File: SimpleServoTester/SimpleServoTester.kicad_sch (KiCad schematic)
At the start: 41 parts, among them J2 Servo, J2 USBASP, J3 OLED, Q1 IRLZ44N, SW1 POWER, SW2 RotaryEncoder_Switch, U1 ATmega328-A, U2 LM7805_TO220, U3 INA219AxD, U4 AMS1117-3.3, Y2 16MHz

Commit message: update
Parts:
- removed C10: 100n/50V, Capacitor_SMD:C_0603_1608Metric, symbol Device:C_Small
- removed RV1: 10k, Footprint:PTV09A-4225F-B502, symbol Device:R_Potentiometer
- added C7, C8: 100n/50V, Capacitor_SMD:C_0603_1608Metric, symbol Device:C_Small
- added R10, R8: 100R, Resistor_SMD:R_0603_1608Metric, symbol Device:R_Small
- H1, H2, H3, H4: footprint MountingHole:MountingHole_3.2mm_M3_Pad_Via -> MountingHole:MountingHole_3.2mm_M3
- SW2: footprint (none) -> Rotary_Encoder:RotaryEncoder_Alps_EC11E-Switch_Vertical_H20mm
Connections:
- net GND: now also SW2.C, C7.1, C8.2
- net at SW2.A: now also R8.2
- net at SW2.B: now also R10.2
- net INT_PIN_2: now reaches U1.1 (PD3)
- net INT_PIN_2: now also C7.2, R8.1
- net DI: now reaches U1.2 (PD4)
- net DI: now also C8.1, R10.1
- no-connect marks 14 -> 12
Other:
- note removed: "POTENTIOMETER"
- moved on the sheet: C15, R9, SW2

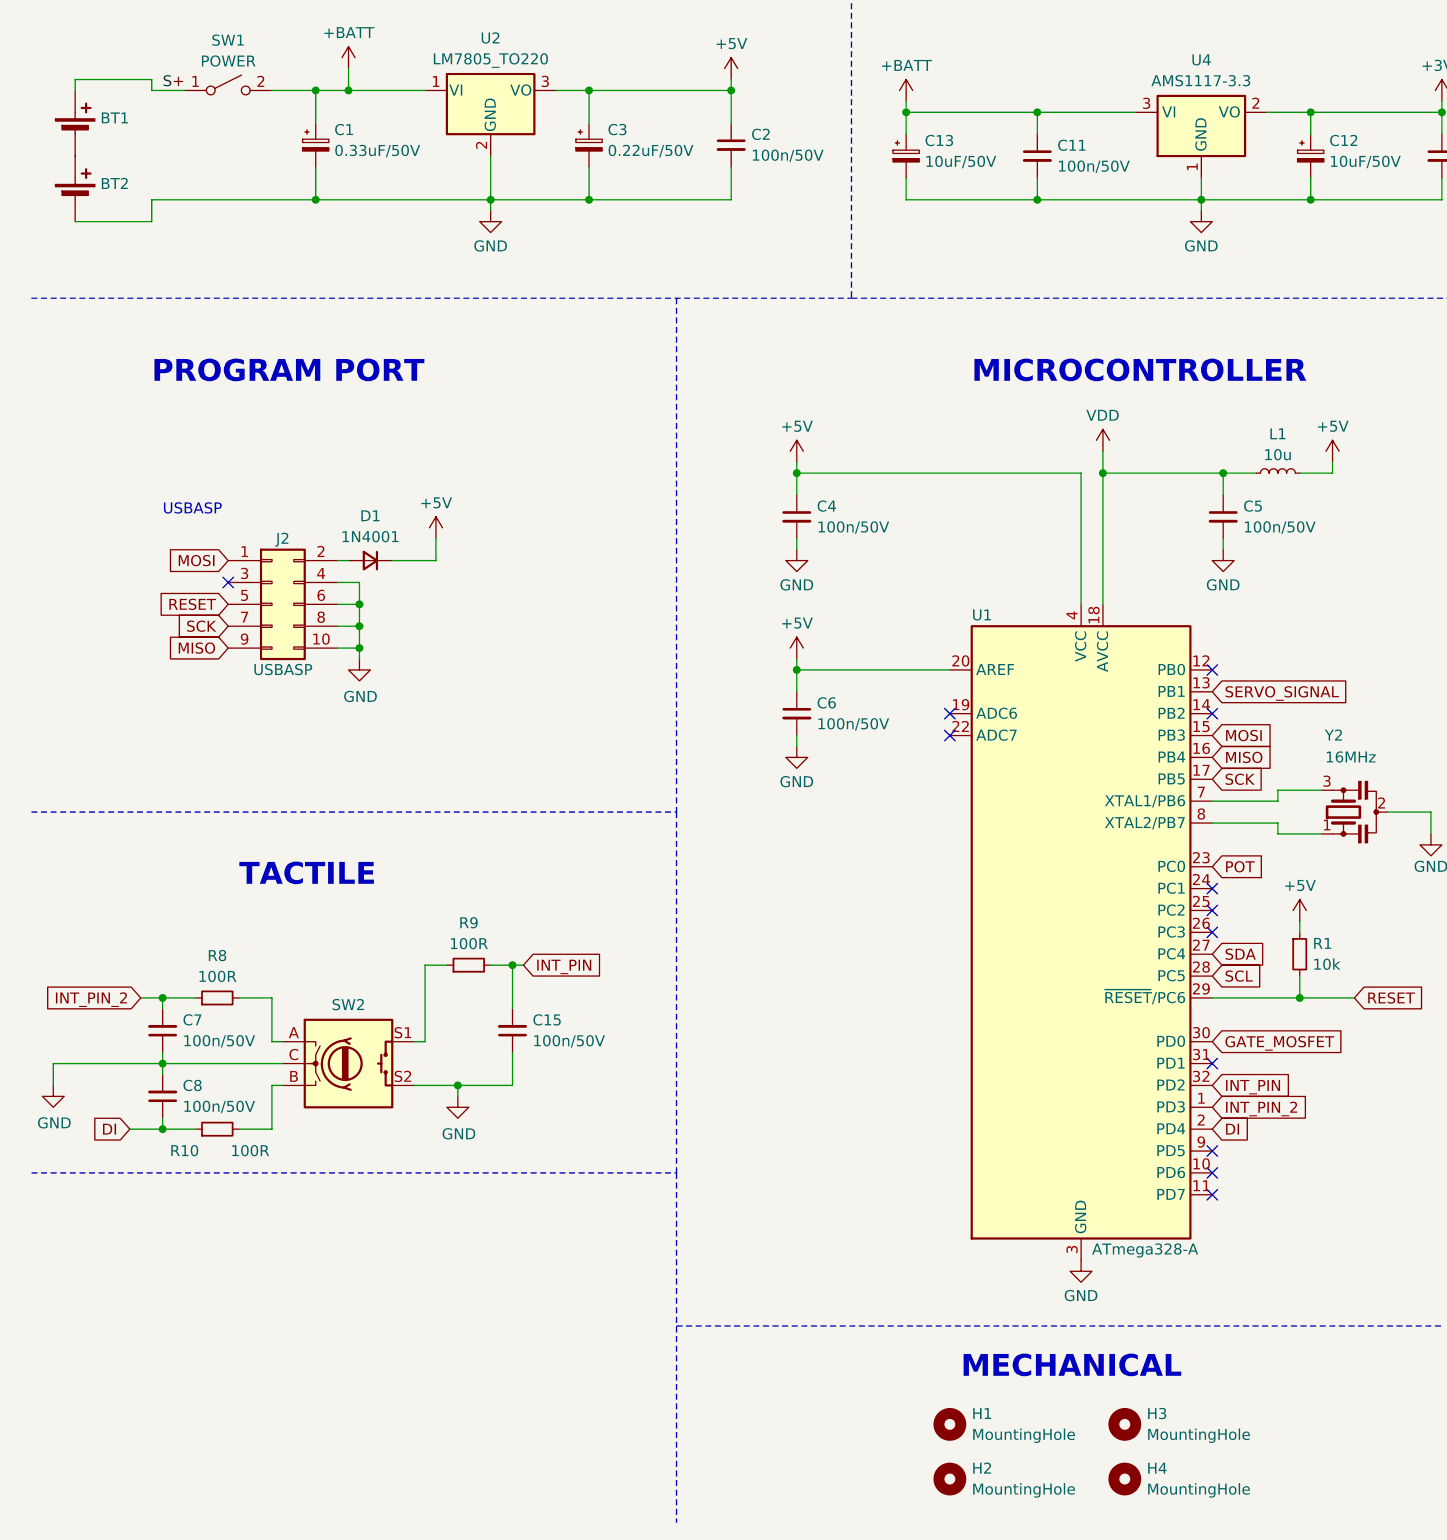
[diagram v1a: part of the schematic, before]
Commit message: update
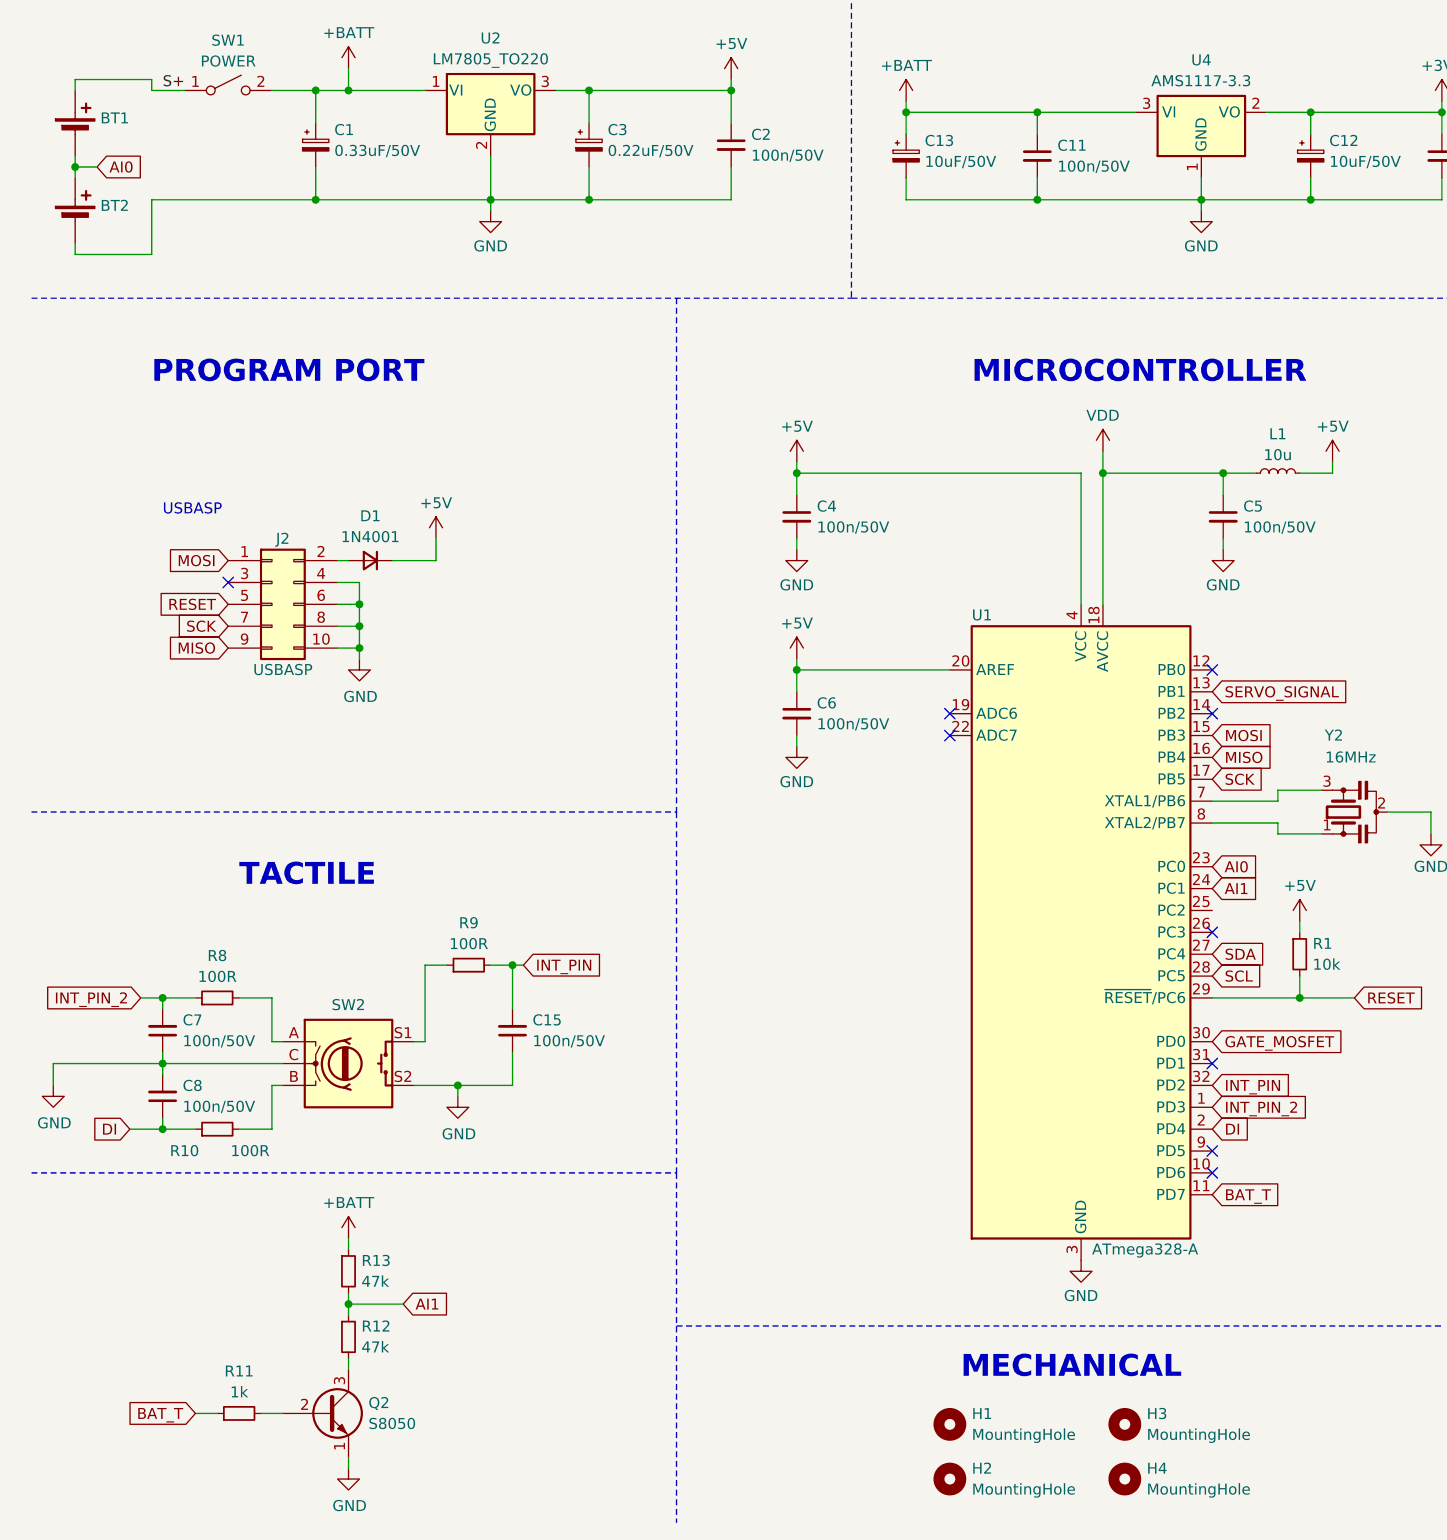
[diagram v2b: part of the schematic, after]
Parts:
- added Q2: S8050, Package_TO_SOT_SMD:SOT-23-3, symbol Transistor_BJT:S8050
- added R11: 1k, Resistor_SMD:R_0603_1608Metric, symbol Device:R_Small
- added R12, R13: 47k, Resistor_SMD:R_0603_1608Metric, symbol Device:R_Small
- R7: footprint Resistor_SMD:R_0603_1608Metric -> Resistor_SMD:R_2512_6332Metric
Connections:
- net POT is gone; now on net AI0: U1.23 (PC0)
- net +BATT: now also R13.1
- net GND: now also Q2.1 (E)
- net AI0: now reaches BT1.2 (-), BT2.1 (+)
- net BAT_T: now reaches U1.11 (PD7)
- net BAT_T: now also R11.1
- net AI1: now reaches U1.24 (PC1)
- net AI1: now also R12.1, R13.2
- new net: Q2.2 (B), R11.2
- new net: Q2.3 (C), R12.2
- no-connect marks 12 -> 9
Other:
- moved on the sheet: BT2

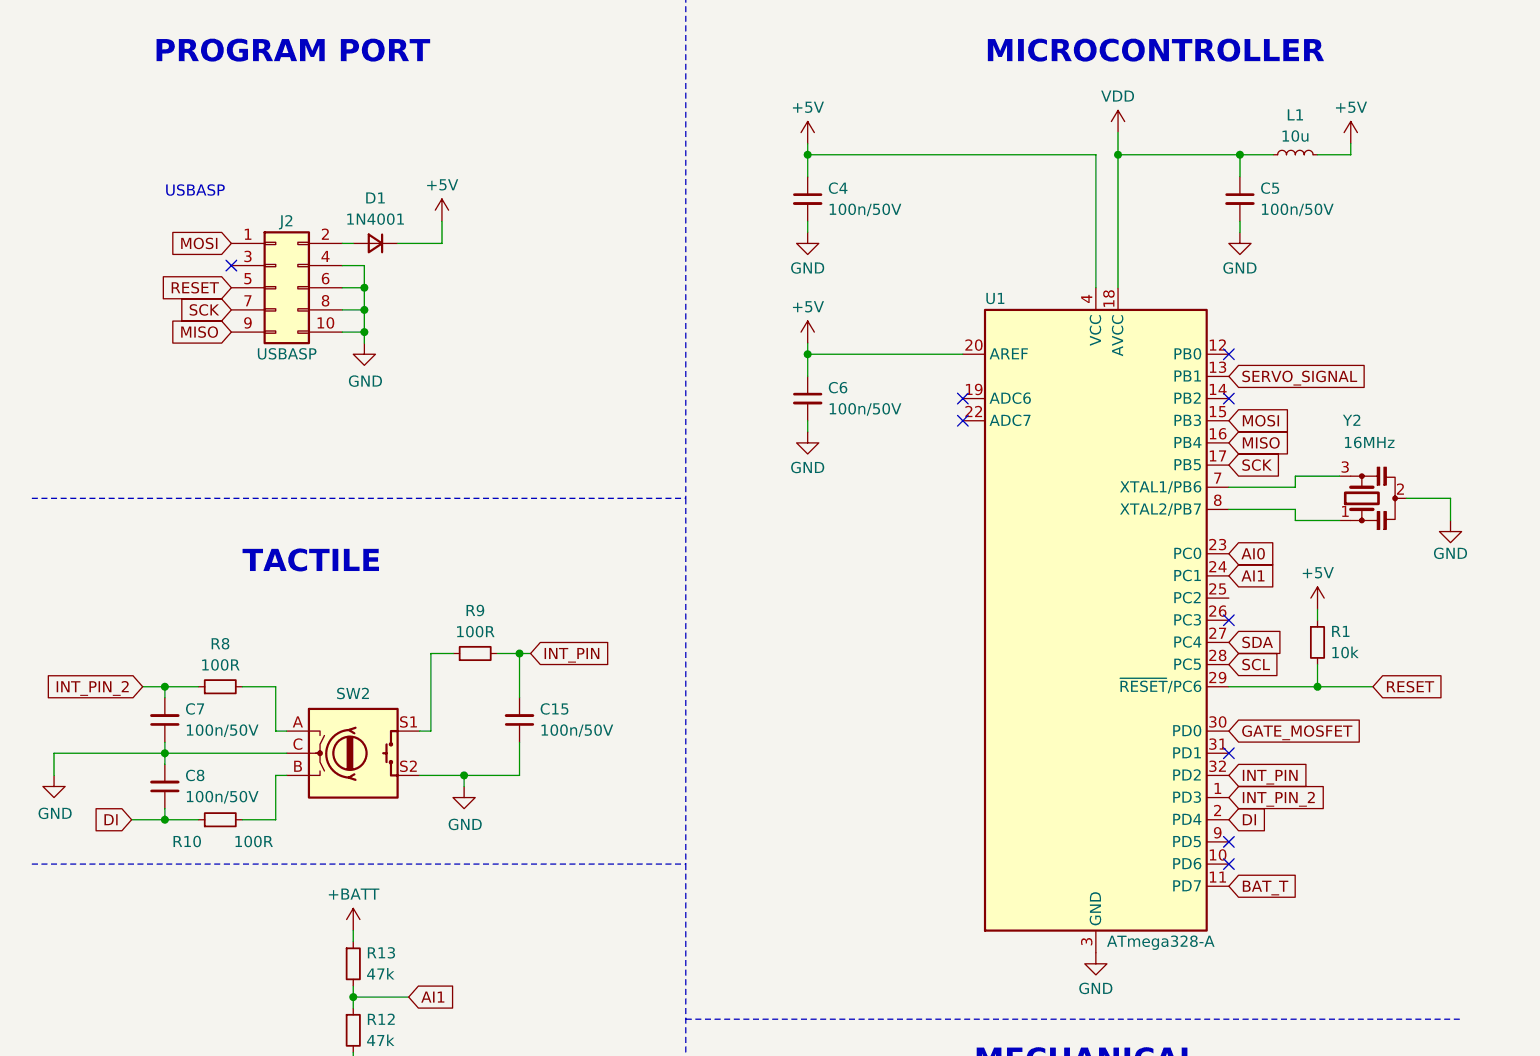
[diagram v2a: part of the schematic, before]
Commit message: update
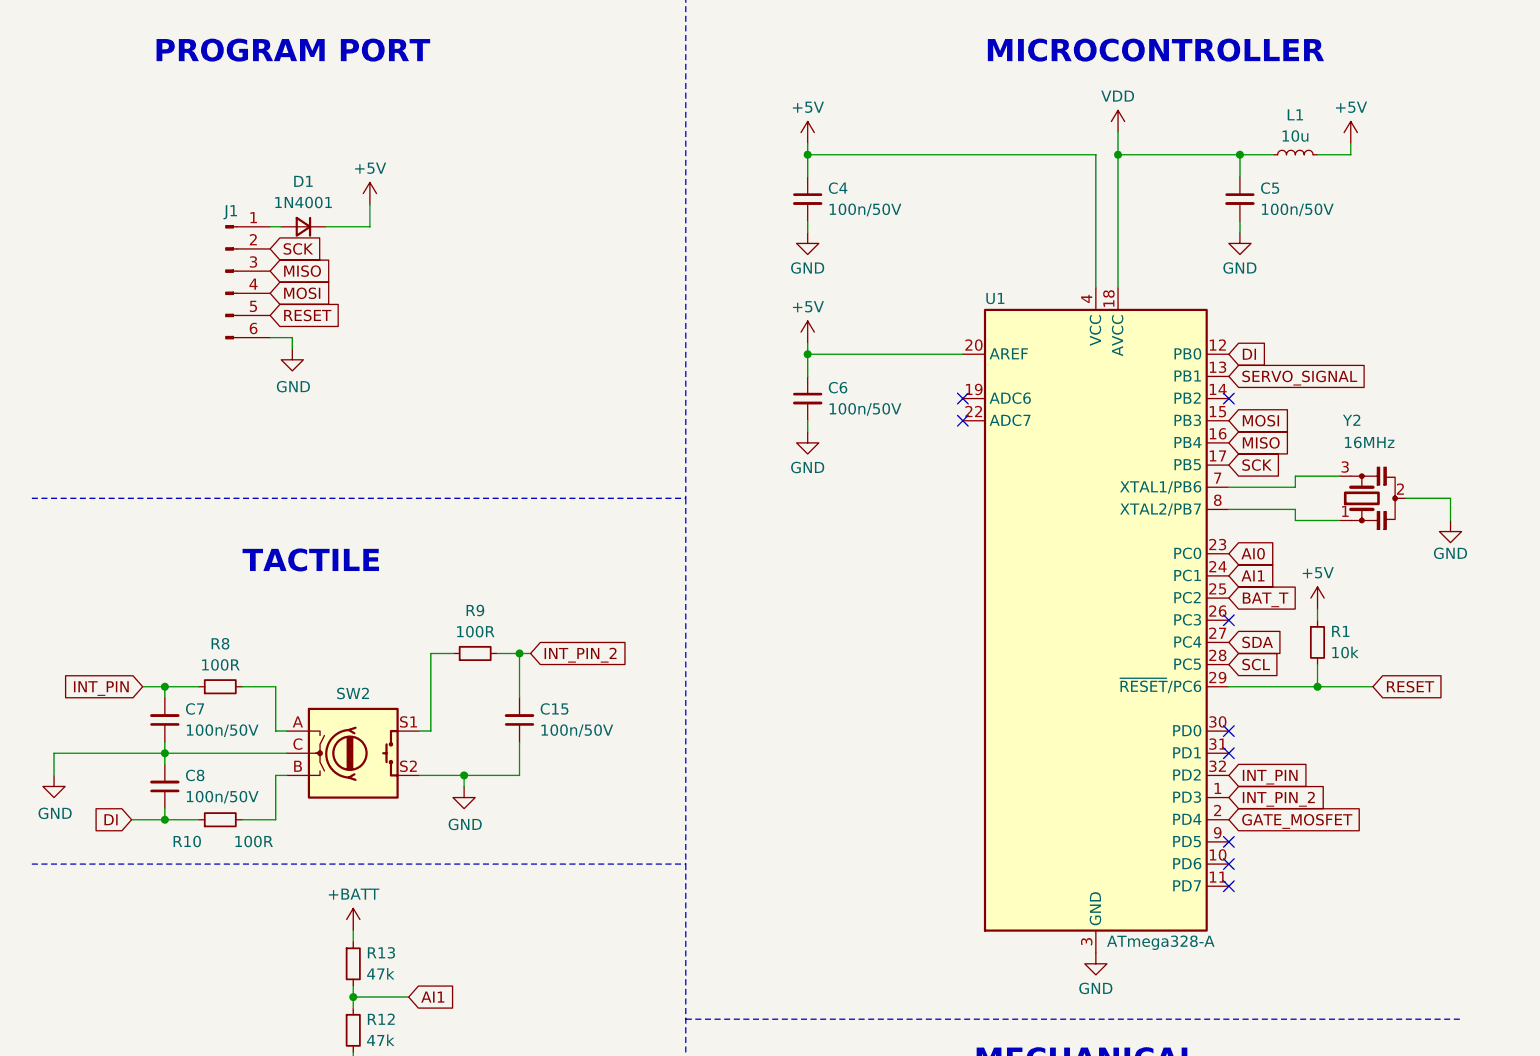
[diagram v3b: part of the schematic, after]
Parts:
- removed J2: USBASP, Connector_IDC:IDC-Header_2x05_P2.54mm_Horizontal, symbol Connector_Generic:Conn_02x05_Odd_Even
- added J1: USBASP, Connector_PinHeader_2.54mm:PinHeader_1x06_P2.54mm_Horizontal, symbol Connector:Conn_01x06_Pin
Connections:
- net BAT_T: now also U1.25 (PC2); no longer U1.11 (PD7)
- net DI: now also U1.12 (PB0); no longer U1.2 (PD4)
- net GATE_MOSFET: now also U1.2 (PD4); no longer U1.30 (PD0)
- net GND: now also J1.6 (Pin_6)
- net INT_PIN: now also C7.2, R8.1; no longer C15.2, R9.2
- net INT_PIN_2: now also C15.2, R9.2; no longer C7.2, R8.1
- net MISO: now also J1.3 (Pin_3)
- net MOSI: now also J1.4 (Pin_4)
- net RESET: now also J1.5 (Pin_5)
- net SCK: now also J1.2 (Pin_2)
- net at D1.2 (A): now also J1.1 (Pin_1)
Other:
- note removed: "USBASP"
- moved on the sheet: D1

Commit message: update
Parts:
- J3: footprint Connector_PinSocket_2.54mm:PinSocket_1x04_P2.54mm_Vertical -> Connector_PinHeader_2.54mm:PinHeader_1x04_P2.54mm_Vertical
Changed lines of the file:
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@@
       (effects (font (size 1.27 1.27)) (justify left))
     )
-    (property "Footprint" "Connector_PinSocket_2.54mm:PinSocket_1x04_P2.54mm_Vertical" (at 218.44 34.29 0)
+    (property "Footprint" "Connector_PinHeader_2.54mm:PinHeader_1x04_P2.54mm_Vertical" (at 218.44 34.29 0)
       (effects (font (size 1.27 1.27)) hide)
     )
